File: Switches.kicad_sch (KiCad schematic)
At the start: 13 parts, among them U4 SN74CBT3126PWR, U5 RS2057XH

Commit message: jlcpcb
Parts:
- C18: MPN (none) -> C565626
- R4: MPN (none) -> C139913
- U4: MPN (none) -> C7142
- U5: MPN (none) -> C255474
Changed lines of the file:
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@@
+      (effects (font (size 1.27 1.27)) hide)
+    )
+    (property "MPN" "C7142" (at 84.455 92.075 0)
       (effects (font (size 1.27 1.27)) hide)
     )
@@
       (effects (font (size 1.27 1.27)) hide)
     )
+    (property "MPN" "C565626" (at 46.99 108.585 0)
+      (effects (font (size 1.27 1.27)) hide)
+    )
     (pin "1")
     (pin "2")
@@
     )
     (property "Datasheet" "DOCUMENTATION" (at 208.28 85.09 0)
+      (effects (font (size 1.27 1.27)) hide)
+    )
+    (property "MPN" "C255474" (at 208.28 80.01 0)
       (effects (font (size 1.27 1.27)) hide)
     )
@@
       (effects (font (size 1.27 1.27)) hide)
     )
+    (property "MPN" "C139913" (at 221.615 102.87 0)
+      (effects (font (size 1.27 1.27)) hide)
+    )

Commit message: routinglogic
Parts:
- U4: JLCRotOffset (none) -> -90
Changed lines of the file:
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@@
+      (effects (font (size 1.27 1.27)) hide)
+    )
+    (property "JLCRotOffset" "-90" (at 84.455 92.075 0)
       (effects (font (size 1.27 1.27)) hide)
     )

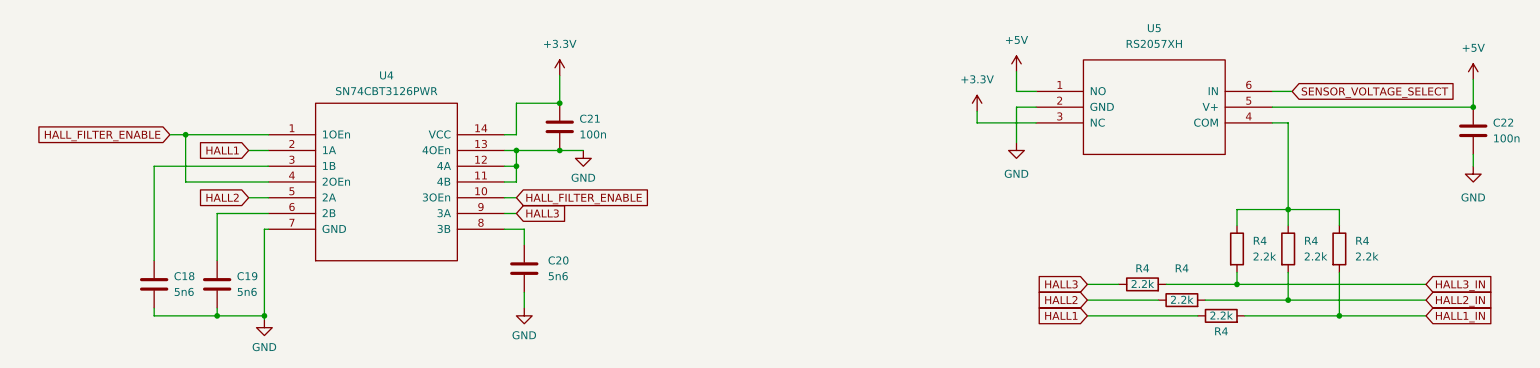
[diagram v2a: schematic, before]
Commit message: routed_again
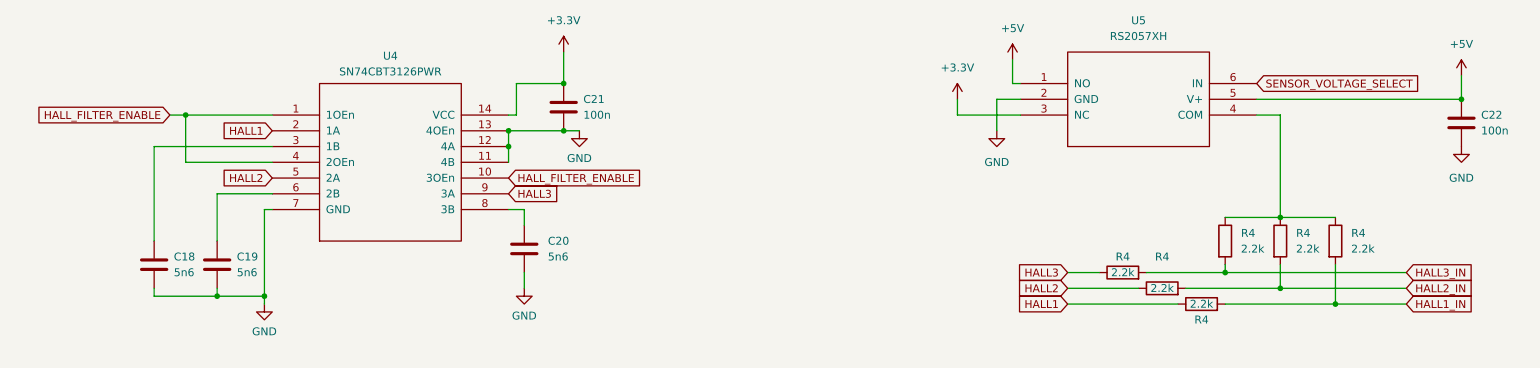
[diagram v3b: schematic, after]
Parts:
- R4: MPN C139913 -> C17520
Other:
- moved on the sheet: C18, C19, C20, C21, C22, R4, U4, U5

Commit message: nearfinish
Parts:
- U5: JLCRotOffset (none) -> -180
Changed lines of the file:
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@@
+      (effects (font (size 1.27 1.27)) hide)
+    )
+    (property "JLCRotOffset" "-180" (at 205.74 78.74 0)
       (effects (font (size 1.27 1.27)) hide)
     )

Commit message: or-gate
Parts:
- R4: MPN (none) -> C17520
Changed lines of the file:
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@@
+      (effects (font (size 1.27 1.27)) hide)
+    )
+    (property "MPN" "C17520" (at 203.2 106.68 90)
       (effects (font (size 1.27 1.27)) hide)
     )
